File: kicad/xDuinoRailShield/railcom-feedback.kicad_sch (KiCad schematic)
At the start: 8 parts, among them Q501 S8050, Q502 S8550, Q503 S8550, Q504 S8050

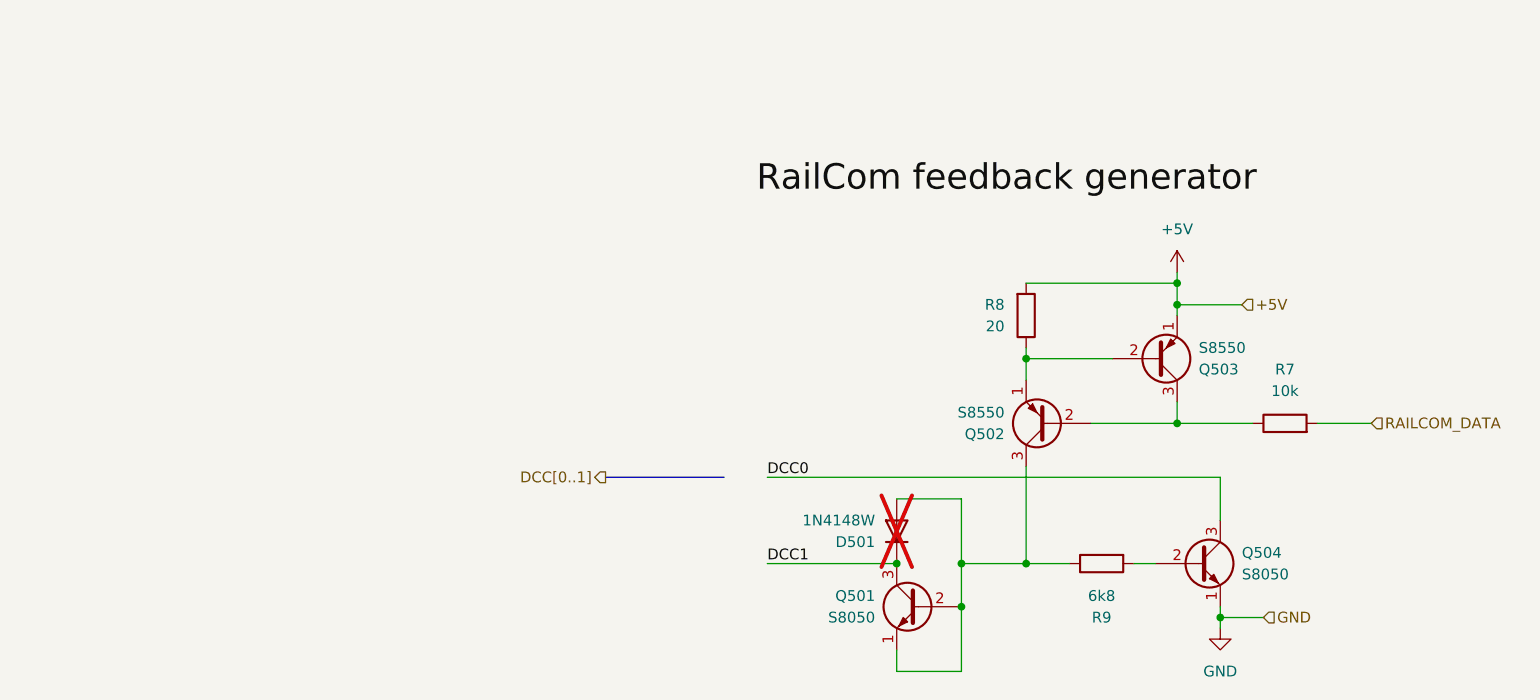
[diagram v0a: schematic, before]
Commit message: A lot of fixes
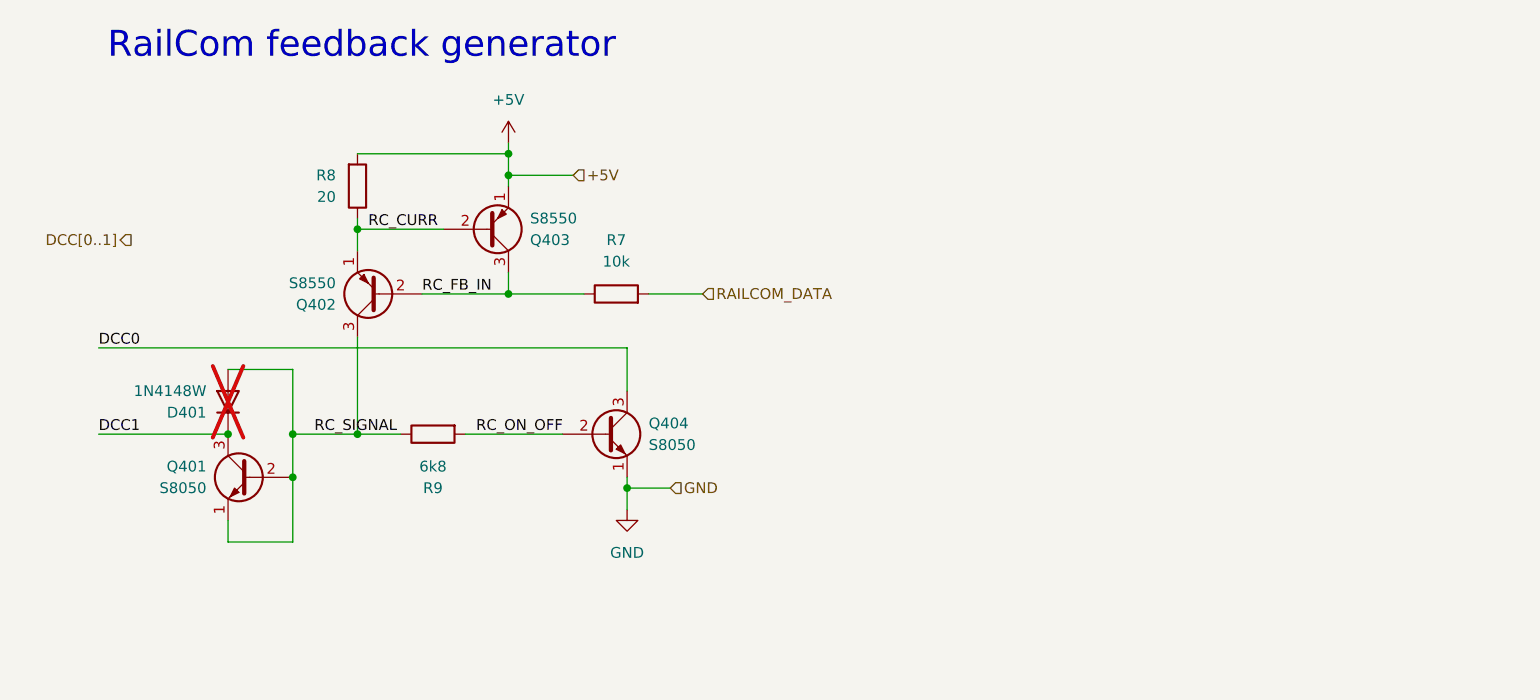
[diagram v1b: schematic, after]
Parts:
- renumbered D501 to D401, Q501 to Q401, Q502 to Q402, Q503 to Q403, Q504 to Q404
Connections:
- net RC_CURR: now reaches Q402.1 (E), Q403.2 (B), R8.1
- net RC_FB_IN: now reaches Q402.2 (B), Q403.3 (C), R7.1
- net RC_SIGNAL: now reaches D401.2 (A), Q401.1 (E), Q401.2 (B), Q402.3 (C), R9.1
- net RC_ON_OFF: now reaches Q404.2 (B), R9.2
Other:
- note added: "RailCom feedback generator"
- moved on the sheet: D401, Q401, Q402, Q403, Q404, R7, R8, R9
